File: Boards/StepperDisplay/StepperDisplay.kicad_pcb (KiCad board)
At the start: 2 copper layers, 94 parts, among them IC1 ATTINY861-P, Q1 BC857, Q10 BC857, Q11 BC857, Q12 BC857, Q13 BC857, Q14 BC857, Q15 BC857, Q16 BC857, Q17 BC857, Q18 BC857, Q2 BC857, Q3 BC857, Q4 BC857, Q5 BC857, Q6 BC857, Q7 BC857, Q8 BC857, Q9 BC857, U1 74HC595, U2 74HC595, U3 ULN2801A, U4 74HC595, U5 74HC595, U6 ULN2801A, U7 74HC595, U8 74HC595, U9 ULN2801A

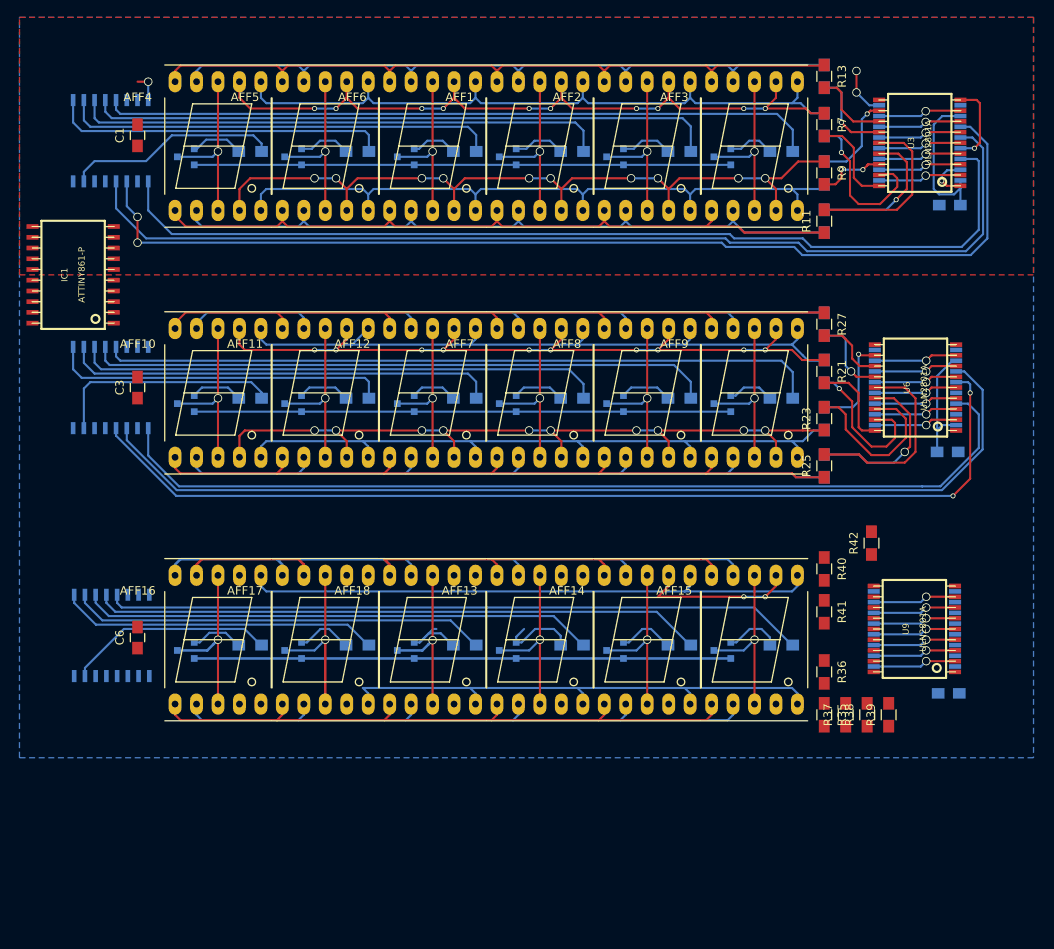
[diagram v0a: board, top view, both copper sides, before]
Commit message: Recover from damaged repository
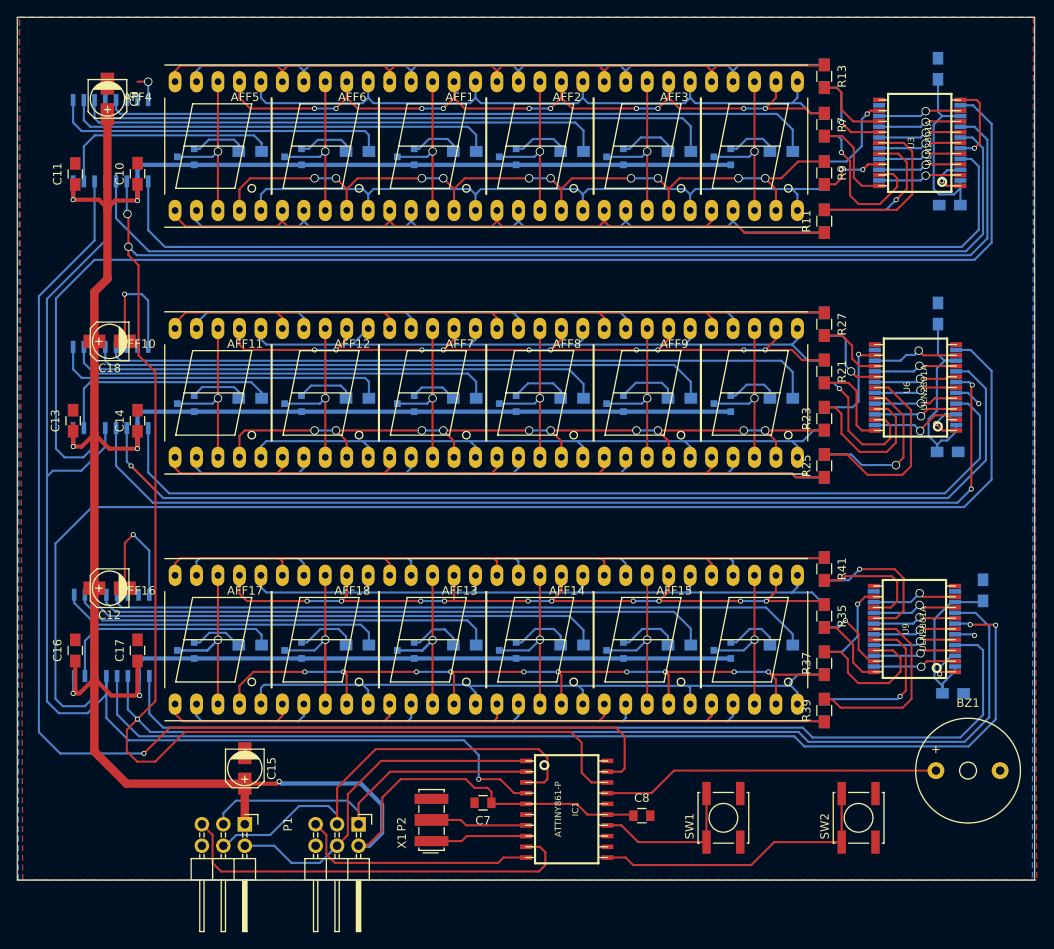
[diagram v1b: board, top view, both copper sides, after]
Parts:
- added BZ1: buzzer, Buzzers_Beepers:Buzzer_12x9.5RM7.6, F.Cu at (179.6, 128.5)
- added C10: 100nF, Capacitors_SMD:C_0805_HandSoldering, F.Cu at (81.3, 57.9)
- added C11: 100nF, Capacitors_SMD:C_0805_HandSoldering, F.Cu at (73.9, 57.9)
- added C12: 100µF, Capacitors_SMD:c_elec_4x5.8, F.Cu at (78.0, 106.9)
- added C13: 100nF, Capacitors_SMD:C_0805_HandSoldering, F.Cu at (73.7, 87.1)
- added C14: 100nF, Capacitors_SMD:C_0805_HandSoldering, F.Cu at (81.3, 87.1)
- added C15: 100µF, Capacitors_SMD:c_elec_4x5.8, F.Cu at (94.0, 128.3)
- added C16: 100nF, Capacitors_SMD:C_0805_HandSoldering, F.Cu at (73.9, 114.3)
- added C17: 100nF, Capacitors_SMD:C_0805_HandSoldering, F.Cu at (81.3, 114.3)
- added C18: 100µF, Capacitors_SMD:c_elec_4x5.8, F.Cu at (78.0, 77.7)
- added C7: 100nF, Capacitors_SMD:C_0805, F.Cu at (122.2, 132.3)
- added C8: 100nF, Capacitors_SMD:C_0805, F.Cu at (141.0, 133.9)
- added C9: 100µF, Capacitors_SMD:c_elec_4x5.8, F.Cu at (77.7, 49.0)
- added P1: CONN_01X06, Pin_Headers:Pin_Header_Angled_2x03, F.Cu at (94.0, 134.9)
- added P2: ISP, Pin_Headers:Pin_Header_Angled_2x03, F.Cu at (107.4, 134.9)
- added SW1: SW_PUSH, Buttons_Switches_SMD:SW_SPST_EVPBF, F.Cu at (150.6, 134.1)
- added SW2: SW_PUSH, Buttons_Switches_SMD:SW_SPST_EVPBF, F.Cu at (166.6, 134.1)
- added X1: CRYSTAL_SMD, Crystals:Resonator_7.2x3mm, F.Cu at (116.1, 134.4)
- C1, C3, C6, R36, R38, R40, R42: moved to B.Cu
- moved C6 100.2 mm to (181.4, 107.2)
- moved C3 95.1 mm to (176.0, 74.4)
- moved C1 95.1 mm to (176.0, 45.5)
- moved IC1 86.1 mm to (132.1, 133.1), turned to 270 degrees
- moved R42 15.3 mm to (162.6, 115.8)
- moved R35 11.7 mm to (162.6, 110.2)
- moved R39 7.64 mm to (162.6, 121.4)
- moved R37 6.60 mm to (162.6, 115.8)
- moved R36 6.60 mm to (162.6, 110.2)
- moved R38 5.11 mm to (162.6, 121.4)
- moved R41 5.08 mm to (162.6, 104.6)
- moved C5 0.51 mm to (177.8, 119.4)
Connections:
- IC1 pad 1: (no net) -> MOSI
- IC1 pad 10: (no net) -> Net-(IC1-Pad10)
- IC1 pad 11: (no net) -> Net-(IC1-Pad11)
- IC1 pad 14: (no net) -> Net-(IC1-Pad14)
- IC1 pad 17: (no net) -> Net-(BZ1-Pad1)
- IC1 pad 2: (no net) -> MISO
- IC1 pad 3: (no net) -> SCK
- IC1 pad 7: (no net) -> Net-(IC1-Pad7)
- IC1 pad 8: (no net) -> Net-(IC1-Pad8)
- IC1 pad 9: (no net) -> CS
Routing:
- net +5V: track 222.8 -> 504.7 mm, vias 0 -> 7
- net /Controller/Ser_Clock: track 243.3 -> 502.4 mm, vias 2 -> 4
- net /LEDsZ/Ser_In: track 0.00 -> 158.3 mm
- net /LEDsY/Ser_In: track 0.00 -> 157.6 mm
- net /LEDsX/Ser_In: track 0.00 -> 146.0 mm, vias 0 -> 1
- net /Controller/Enable: track 0.00 -> 145.7 mm, vias 0 -> 1
- net /LEDsZ/R_Clock: track 0.00 -> 127.5 mm, vias 0 -> 2
- net Net-(U7-Pad9): track 0.00 -> 116.6 mm
- net Net-(AFF13-Pad4): track 0.00 -> 92.2 mm, vias 0 -> 10
- net Net-(AFF13-Pad7): track 18.8 -> 88.9 mm, vias 2 -> 10
- net SCK: track 0.00 -> 53.7 mm
- net CS: track 0.00 -> 49.3 mm
- net MISO: track 0.00 -> 43.8 mm
- net MOSI: track 0.00 -> 42.0 mm
- net Net-(BZ1-Pad1): track 0.00 -> 40.0 mm
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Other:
- board outline added: 120.4 x 102.1 mm
